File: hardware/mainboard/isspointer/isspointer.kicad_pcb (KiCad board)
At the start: 2 copper layers, 132.7 x 75.6 mm, 110 parts, among them J1 USB_B_Micro, J2 Motor 1, J3 Motor 2, J4 U_FL-R-SMT-1_10_, Q1 SS8050-G, Q2 SS8050-G, Q3 DMN67D8L, Q4 DMN67D8L, SW1 Boot, SW2 Reset, SW3 Up, SW4 Select, SW5 Down, U1 AMS1117-3.3, U10 NEO-6M-0-001, U11 24AA32-OT, U2 CP2102N-A01-GQFN28, U3 esp32-WROOM-32D, U4 DRV8834_HTSSOP, U5 DRV8834_HTSSOP, U6 LSM303DLHC, U7 EE-SX3350, U8 EE-SX3350, U9 CFAL12864N

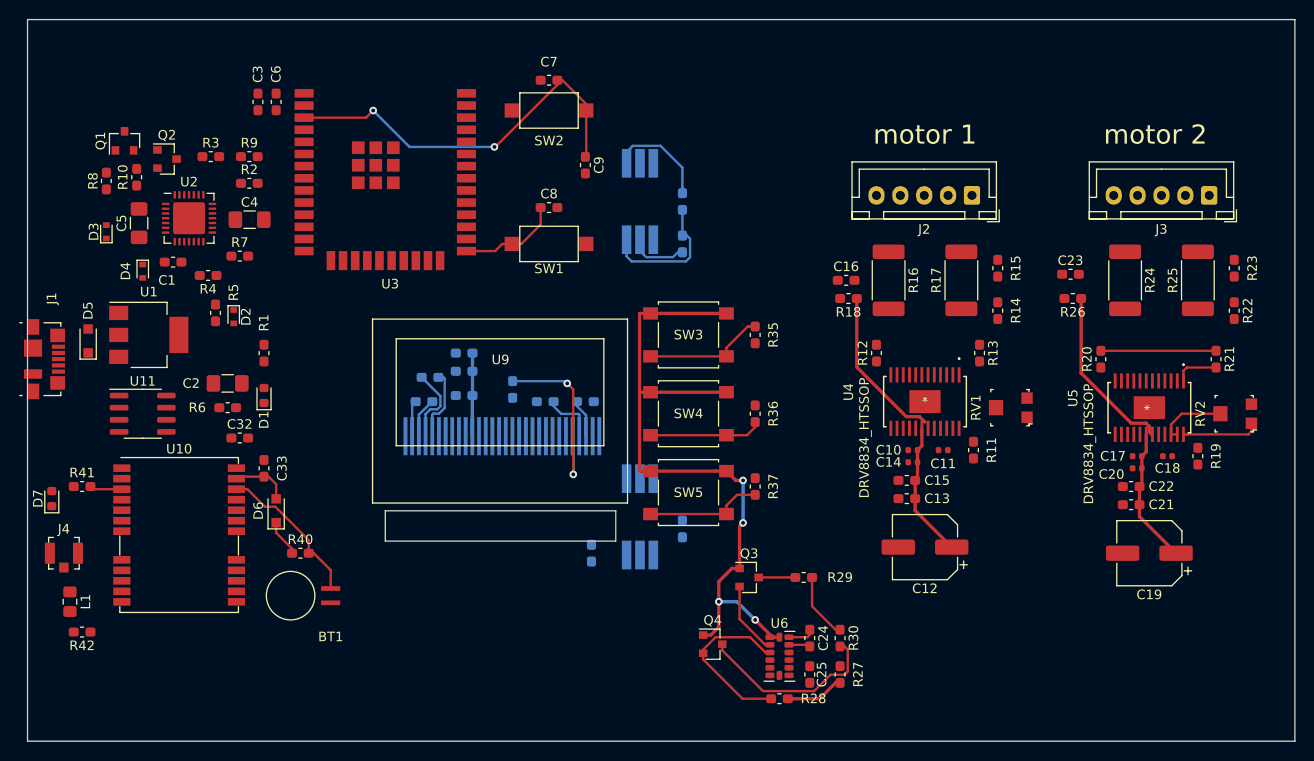
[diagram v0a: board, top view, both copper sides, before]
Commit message: work MITAI bluetooth connection
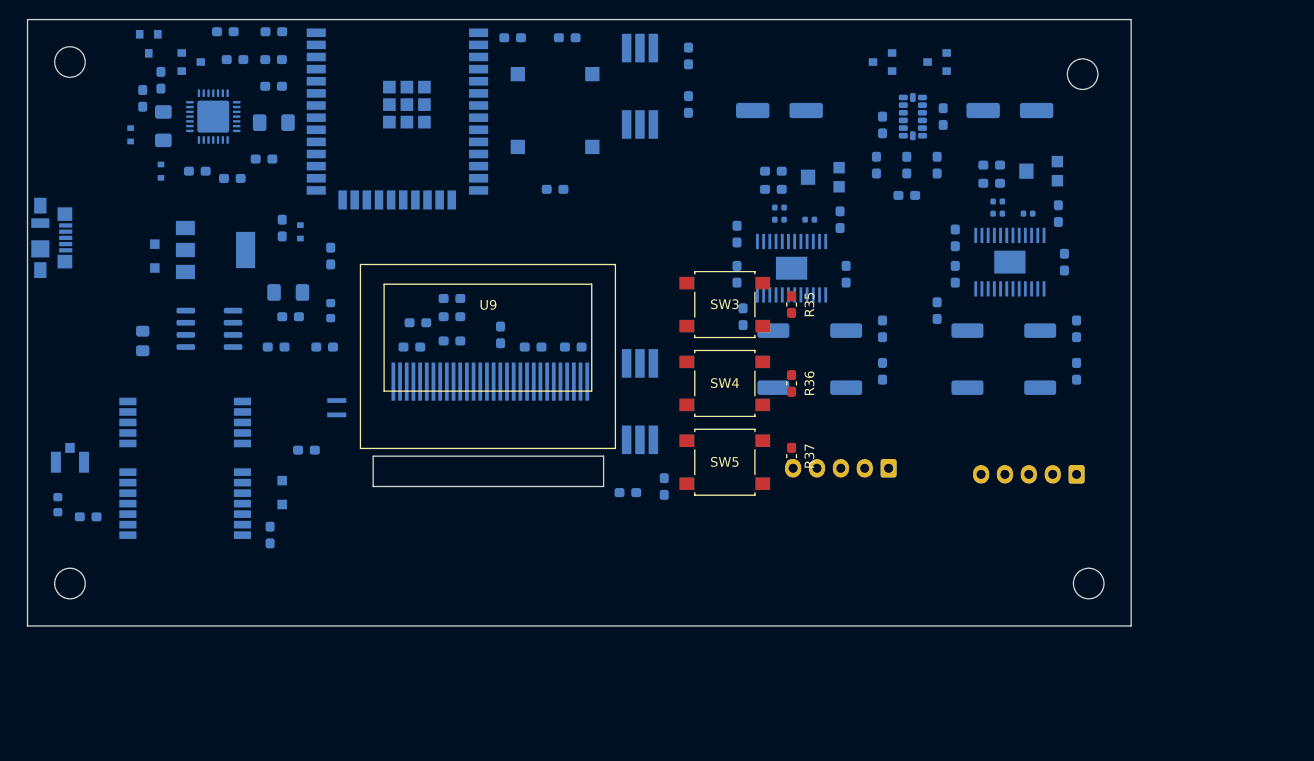
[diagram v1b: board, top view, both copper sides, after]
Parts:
- added REF**: MountingHole_3.2mm_M3, MountingHole:MountingHole_3.2mm_M3, F.Cu at (51.4, 85.1)
- added REF**: MountingHole_3.2mm_M3, MountingHole:MountingHole_3.2mm_M3, F.Cu at (158.1, 85.1)
- added REF**: MountingHole_3.2mm_M3, MountingHole:MountingHole_3.2mm_M3, F.Cu at (157.5, 31.8)
- added REF**: MountingHole_3.2mm_M3, MountingHole:MountingHole_3.2mm_M3, F.Cu at (51.4, 30.5)
- BT1, C1, C10, C11, C12, C13, C14, C15, C16, C17, C18, C19, C2, C20, C21, C22, C23, C24, C25, C3, C32, C33, C4, C5, C6, C7, C8, C9, D1, D2, D3, D4, D5, D6, D7, J1, J2, J3, J4, L1, Q1, Q2, Q3, Q4, R1, R10, R11, R12, R13, R14, R15, R16, R17, R18, R19, R2, R20, R21, R22, R23, R24, R25, R26, R27, R28, R29, R3, R30, R4, R40, R41, R42, R5, R6, R7, R8, R9, RV1, RV2, SW1, SW2, U1, U10, U11, U2, U3, U4, U5, U6: moved to B.Cu
- moved Q4 65.3 mm to (142.2, 30.5), turned to 180 degrees
- moved U6 58.2 mm to (139.7, 36.2), turned to 180 degrees
- moved Q3 55.8 mm to (136.5, 30.5), turned to 180 degrees
- moved C25 55.0 mm to (142.2, 41.3)
- moved R28 54.4 mm to (139.1, 44.5), turned to 0 degrees
- moved C24 54.3 mm to (136.5, 37.1)
- moved R27 53.5 mm to (135.9, 41.3)
- moved R29 50.4 mm to (142.9, 36.2), turned to 90 degrees
- moved R30 50.0 mm to (139.1, 41.3)
- moved C19 48.6 mm to (149.9, 35.6)
- moved C12 48.2 mm to (125.7, 35.6)
- moved C21 38.4 mm to (148.0, 41.3)
- moved C13 37.0 mm to (125.1, 41.9)
- moved R42 36.1 mm to (73.0, 60.3)
- moved C22 34.9 mm to (148.0, 43.2)
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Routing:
- net +3V3: track 93.8 -> 0.00 mm, vias 4 -> 0
- net VBUS: track 63.6 -> 0.00 mm
- net /EN: track 41.2 -> 0.00 mm, vias 2 -> 0
- net +5V: track 21.3 -> 0.00 mm
- net /IO21: track 19.6 -> 0.00 mm
- net Net-(R38-Pad1): track 19.6 -> 0.00 mm, vias 2 -> 0
- net /SDALV: track 18.0 -> 0.00 mm
- net Net-(BT1-Pad1): track 16.1 -> 0.00 mm
- net /BTN_UP: track 12.8 -> 0.00 mm
- net /BTN_DOWN: track 12.3 -> 0.00 mm
- net Net-(R20-Pad2): track 12.1 -> 0.00 mm
- net /BTN_SELECT: track 11.8 -> 0.00 mm
- net Net-(R31-Pad1): track 10.9 -> 0.00 mm
- net /IO0: track 10.7 -> 0.00 mm
- net Net-(RV2-Pad1): track 8.10 -> 0.00 mm
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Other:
- board size 132.7 x 75.6 mm -> 115.6 x 63.5 mm
